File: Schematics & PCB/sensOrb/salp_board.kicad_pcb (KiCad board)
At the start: 2 copper layers, 57 parts, among them J1 ATTINY3226, J10 POWER, J4 Conn_01x03, J8 ATTINY3226, J9 POWER_JUMPER, Q1 IRLML6402, Q2 IRLML6402, SW1 SW_DIP_x02, SW2 SW_DPDT_x2, U1 LD1117S33TR, U2 PN5321A3HN/C106_55, U3 ATtiny3226-S, U4 TP4057, U6 DW01A, Y1 27.12 MHz

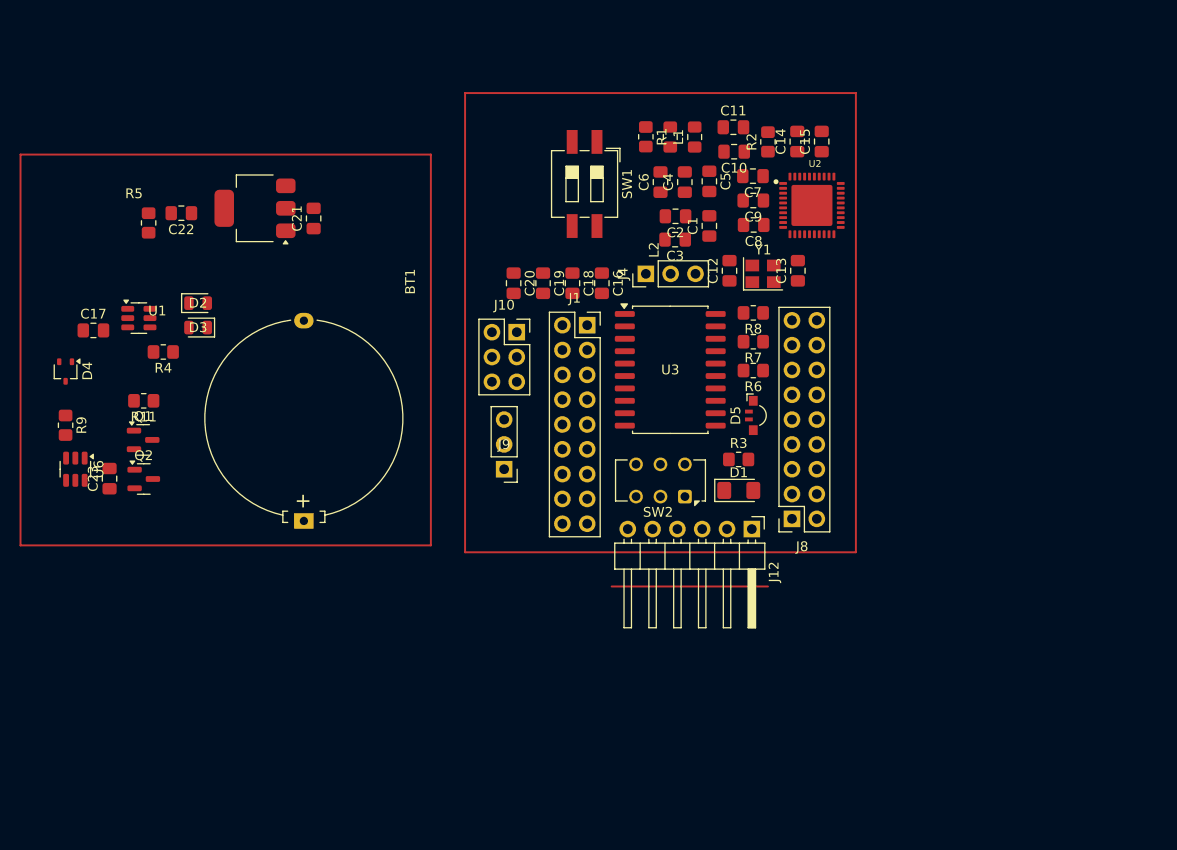
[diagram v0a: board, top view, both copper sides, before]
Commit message: Layout 1: No ERC/DRC done yet
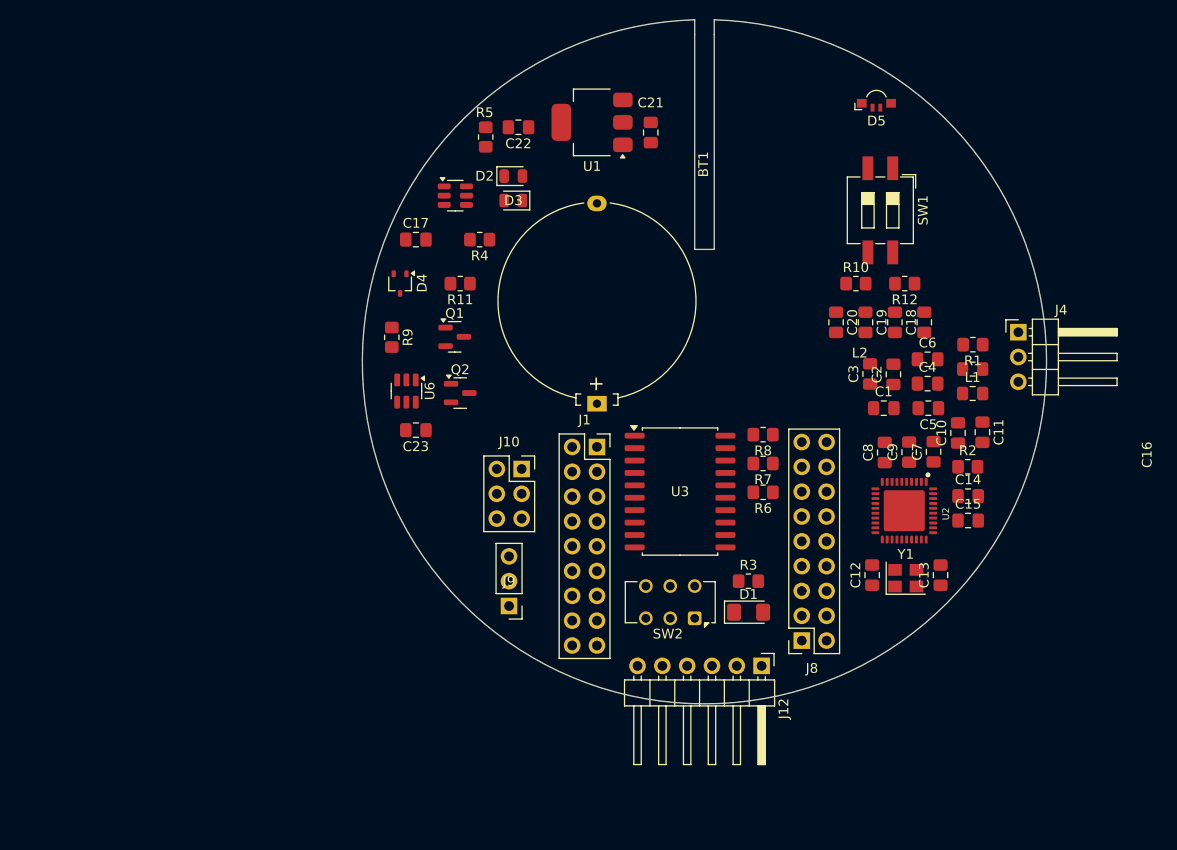
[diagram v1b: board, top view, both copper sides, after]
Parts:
- added R10: 1k, Resistor_SMD:R_0805_2012Metric_Pad1.20x1.40mm_HandSolder, F.Cu at (195.5, 66.5)
- added R12: 1k, Resistor_SMD:R_0805_2012Metric_Pad1.20x1.40mm_HandSolder, F.Cu at (200.5, 66.5)
- J4: footprint Connector_PinHeader_2.54mm:PinHeader_1x03_P2.54mm_Vertical -> Connector_PinHeader_2.54mm:PinHeader_1x03_P2.54mm_Horizontal
- moved C15 41.6 mm to (207.0, 90.8), turned to 0 degrees
- moved C11 40.3 mm to (208.4, 81.7), turned to -90 degrees
- moved C14 40.3 mm to (207.0, 88.2), turned to 0 degrees
- moved R1 39.7 mm to (207.5, 72.8), turned to 180 degrees
- moved R2 39.0 mm to (206.9, 85.2), turned to 0 degrees
- moved L2 39.0 mm to (207.4, 75.2), turned to 0 degrees
- moved L1 38.7 mm to (207.4, 77.8), turned to 0 degrees
- moved J4 38.6 mm to (212.1, 71.5), turned to 0 degrees
- moved C10 36.8 mm to (205.9, 81.8), turned to 90 degrees
- moved C21 35.6 mm to (174.5, 51.0)
- moved C22 35.6 mm to (161.0, 50.5)
- moved U1 35.6 mm to (168.5, 50.0)
- moved R5 35.6 mm to (157.6, 51.5)
- moved D4 35.4 mm to (148.8, 66.5)
- moved U6 34.8 mm to (149.5, 77.5)
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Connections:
- C1 pad 1: Net-(J4-Pin_3) -> Net-(J4-Pin_1)
- C1 pad 2: Net-(J4-Pin_2) -> Net-(J4-Pin_1)
- C14 pad 1: /DVDD -> +3.3V
- C15 pad 1: /DVDD -> +3.3V
- C16 pad 1: GND -> VCC
- C18 pad 1: GND -> VCC
- C19 pad 1: GND -> VCC
- C2 pad 1: Net-(J4-Pin_2) -> Net-(J4-Pin_1)
- C21 pad 1: GND -> VCC
- C3 pad 1: Net-(J4-Pin_3) -> Net-(J4-Pin_1)
- C5 pad 2: Net-(J4-Pin_2) -> Net-(J4-Pin_1)
- C6 pad 1: Net-(J4-Pin_2) -> Net-(J4-Pin_1)
- C7 pad 1: /TVDD -> +3.3V
- C8 pad 1: /AVDD -> +3.3V
- C9 pad 1: /TVDD -> +3.3V
- D4 pad 2: /V_REG -> /V_USB
- J10 pad 1: GND -> VCC
- J10 pad 4: GND -> +3.3V
- J10 pad 5: +3.3V -> GND
- J4 pad 2: Net-(J4-Pin_2) -> Net-(J4-Pin_1)
- J4 pad 3: Net-(J4-Pin_3) -> Net-(J4-Pin_1)
- J9 pad 1: /V_USB -> GND
- Q2 pad 3: GND -> VCC
- SW1 pad 1: /DVDD -> +3.3V
- SW1 pad 2: /DVDD -> +3.3V
- SW1 pad 3: GND -> /I1
- SW1 pad 4: GND -> /IO
- U1 pad 3: GND -> VCC
- U2 pad 11: /AVSS -> GND
- U2 pad 16: GND -> /IO
- U2 pad 17: GND -> /I1
- U2 pad 23: GND -> VCC
- U2 pad 25: /IRQ -> /PA7
- U2 pad 26: /RSTOUT_N -> unconnected-(U2-RSTOUT_N-Pad26)
- U2 pad 31: /DEBUG_TX -> unconnected-(U2-P31/UART_TX-Pad31)
- U2 pad 39: /DVDD -> +3.3V
- U2 pad 5: /TVDD -> +3.3V
- U2 pad 8: /AVDD -> +3.3V
- U3 pad 1: GND -> VCC
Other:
- board outline added: 70 x 70 mm

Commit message: Semi-finalized PCB design
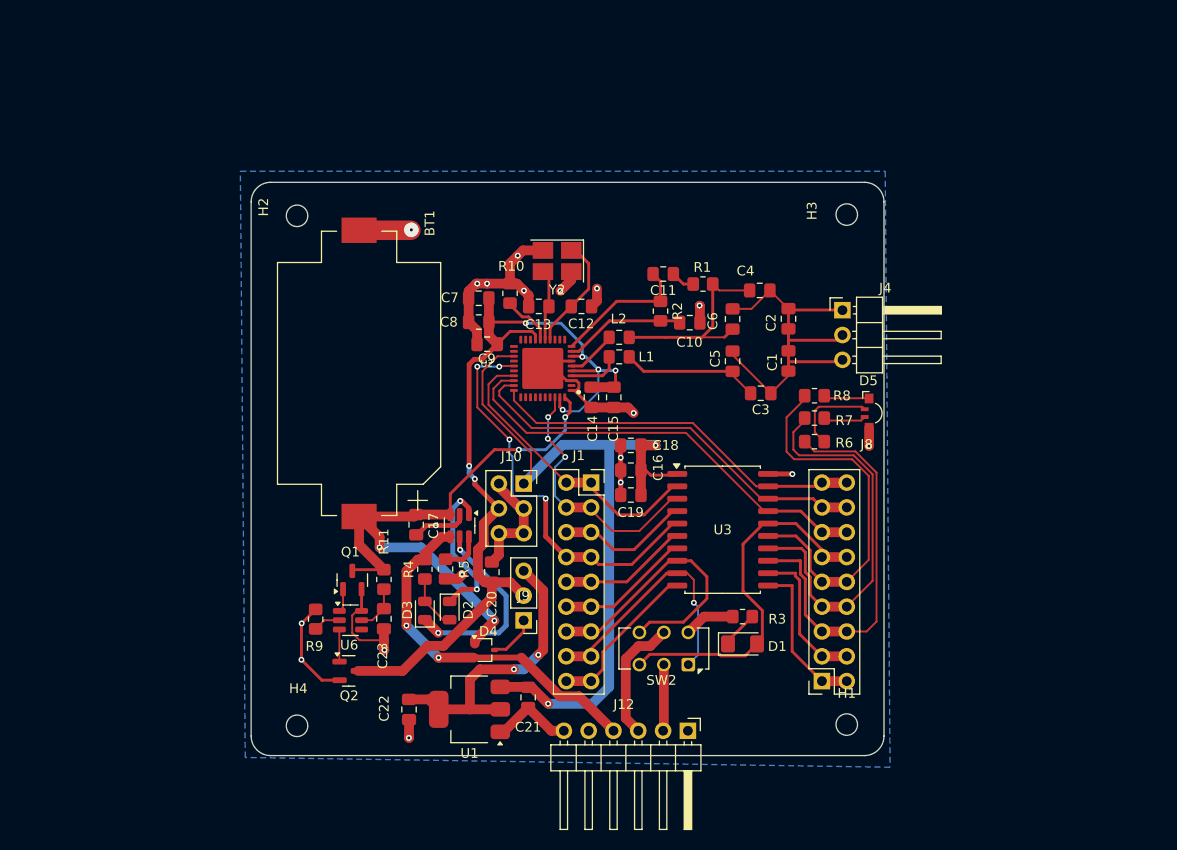
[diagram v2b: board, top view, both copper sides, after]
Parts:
- removed R12: 1k, Resistor_SMD:R_0805_2012Metric_Pad1.20x1.40mm_HandSolder
- removed SW1: SW_DIP_x02, Button_Switch_SMD:SW_DIP_SPSTx02_Slide_6.7x6.64mm_W8.61mm_P2.54mm_LowProfile
- removed Y1: 27.12 MHz, Crystal:Crystal_SMD_3225-4Pin_3.2x2.5mm
- added H1: MountingHole, MountingHole:MountingHole_2.2mm_M2, F.Cu at (194.6, 111.6)
- added H2: MountingHole, MountingHole:MountingHole_2.2mm_M2, F.Cu at (138.3, 59.6)
- added H3: MountingHole, MountingHole:MountingHole_2.2mm_M2, F.Cu at (194.6, 59.4)
- added H4: MountingHole, MountingHole:MountingHole_2.2mm_M2, F.Cu at (138.3, 111.8)
- added Y2: 27.12 MHz, Crystal:Crystal_SMD_SeikoEpson_TSX3225-4Pin_3.2x2.5mm_HandSoldering, F.Cu at (164.9, 64.2)
- BT1: footprint Battery:Battery_Panasonic_CR2032-HFN_Horizontal_CircularHoles -> Battery:BatteryHolder_Keystone_1060_1x2032
- moved U1 61.4 mm to (156.0, 110.1)
- moved C22 60.6 mm to (149.8, 110.1), turned to -90 degrees
- moved C21 59.2 mm to (162.0, 108.9), turned to -90 degrees
- moved C13 49.5 mm to (163.0, 68.8), turned to 180 degrees
- moved C7 49.1 mm to (156.9, 68.0), turned to 180 degrees
- moved D2 44.9 mm to (153.9, 100.0), turned to -90 degrees
- moved C9 44.6 mm to (157.8, 72.7), turned to 180 degrees
- moved R5 44.4 mm to (153.5, 95.7), turned to 90 degrees
- moved C8 43.6 mm to (156.9, 70.4), turned to 180 degrees
- moved C20 43.5 mm to (158.2, 96.0), turned to 90 degrees
- moved D3 42.9 mm to (151.4, 100.0), turned to 90 degrees
- moved C12 40.5 mm to (167.4, 68.8), turned to 0 degrees
- moved C14 39.9 mm to (168.4, 78.1), turned to -90 degrees
- moved U2 39.8 mm to (163.4, 75.2), turned to 180 degrees
- moved D4 38.5 mm to (157.5, 104.0), turned to 0 degrees
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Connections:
- D4 pad 3: GND -> /VOR
- J9 pad 1: GND -> /VOR
- Q2 pad 3: VCC -> +3.3V
- R10 pad 2: /I1 -> Net-(U2-I0)
- U2 pad 16: /IO -> Net-(U2-I0)
- U2 pad 17: /I1 -> +3.3V
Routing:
- net GND: track 0.00 -> 108.3 mm, vias 0 -> 19
- net +3.3V: track 0.00 -> 93.6 mm, vias 0 -> 7
- net VCC: track 0.00 -> 80.6 mm, vias 0 -> 2
- net +BAT: track 0.00 -> 74.5 mm, vias 0 -> 4
- net /PA1: track 0.00 -> 45.4 mm
- net /PA2: track 0.00 -> 42.5 mm
- net /PA7: track 0.00 -> 42.2 mm, vias 0 -> 4
- net /PA3: track 0.00 -> 41.4 mm
- net /PC1: track 0.00 -> 41.4 mm
- net Net-(J4-Pin_1): track 0.00 -> 40.6 mm
- net /PC2: track 0.00 -> 40.1 mm
- net /PC3: track 0.00 -> 38.6 mm
- net /V_USB: track 0.00 -> 37.8 mm, vias 0 -> 2
- net /PA0: track 0.00 -> 37.7 mm
- net /PA4: track 0.00 -> 30.6 mm
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- added copper zone on B.Cu, net GND
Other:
- board size 70 x 70 mm -> 64.8 x 58.7 mm
